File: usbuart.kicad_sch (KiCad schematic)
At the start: 15 parts, among them J7 USB_C_Receptacle_PowerOnly_6P, U1 CH224K

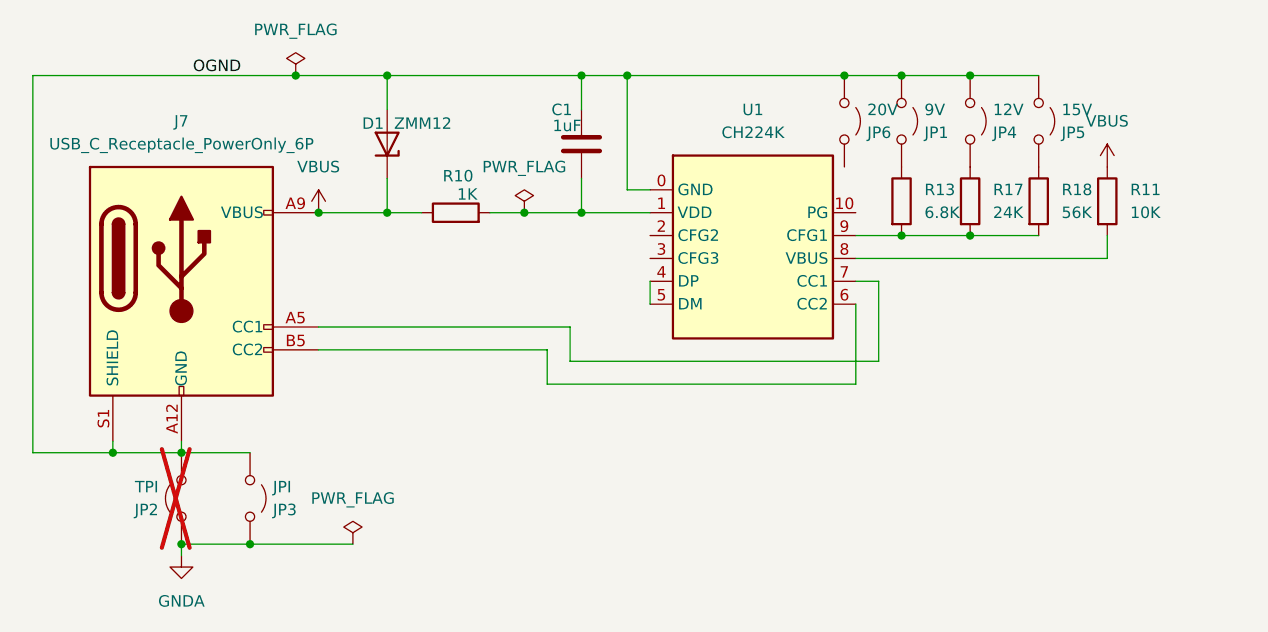
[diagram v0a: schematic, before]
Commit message: Update
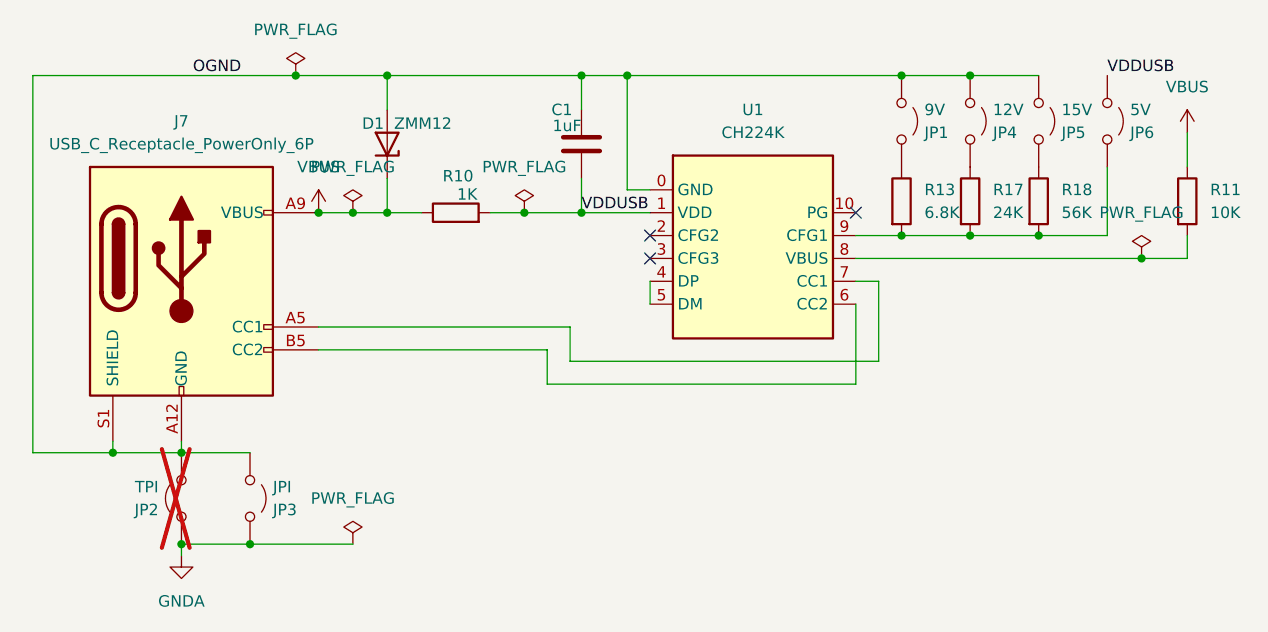
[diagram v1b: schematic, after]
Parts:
- removed U1: CH224K, Package_SO:SSOP-10-1EP_3.9x4.9mm_P1mm_EP2.1x3.3mm_ThermalVias, symbol MCU_NXP_M2:CH224K
- added U1: CH224K, Package_SO:SSOP-10-1EP_3.9x4.9mm_P1mm_EP2.1x3.3mm_ThermalVias, symbol MCU_NXP_S32M2:CH224K
- J7: footprint (none) -> Connector_USB:USB_C_Receptacle_GCT_USB4125-xx-x_6P_TopMnt_Horizontal
- JP6: value 20V -> 5V
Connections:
- net OGND: now also U1.0 (GND); no longer JP6.2 (B)
- net VDDUSB: now reaches C1.1, R10.2
- net VDDUSB: now also JP6.2 (B), U1.1 (VDD)
- net at R13.2, R17.2, R18.2: now also JP6.1 (A), U1.9 (CFG1)
- net at J7.A5 (CC1): now also U1.7 (CC1)
- net at J7.B5 (CC2): now also U1.6 (CC2)
- net at R11.2: now also U1.8 (VBUS)
- new net: U1.4 (DP), U1.5 (DM)
- no-connect marks 0 -> 3
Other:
- moved on the sheet: R11
